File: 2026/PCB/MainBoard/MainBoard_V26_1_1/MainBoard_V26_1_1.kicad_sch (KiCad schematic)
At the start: 87 parts, among them J1 Raspberry_Pi_2_3, J13 //Drib, J15 TFT3, J16 CAN_CON, J2 fan, J4 metor, J6 Debug, J8 MOLEX MINISPOX, Q1 Q_NMOS_GSD, Q2 Q_NMOS_GSD, SW1 SW_MEC_5E, SW2 Ras_1, SW3 Ras_2, SW4 SW_Wuerth_450301014042, SW5 SW_MEC_5E, SW6 SW_MEC_5E, U1 STM32F446RETx, U10 MPU9250, U2 LMR51460FSQDRRRQ1, U3 MOUDLE-SEEEDUINO-XIAO, U5 MCP1703AT-3302E/CB, U6 BNO055, U8 MAX3051, Y1 CSTNE16M0V530000R0

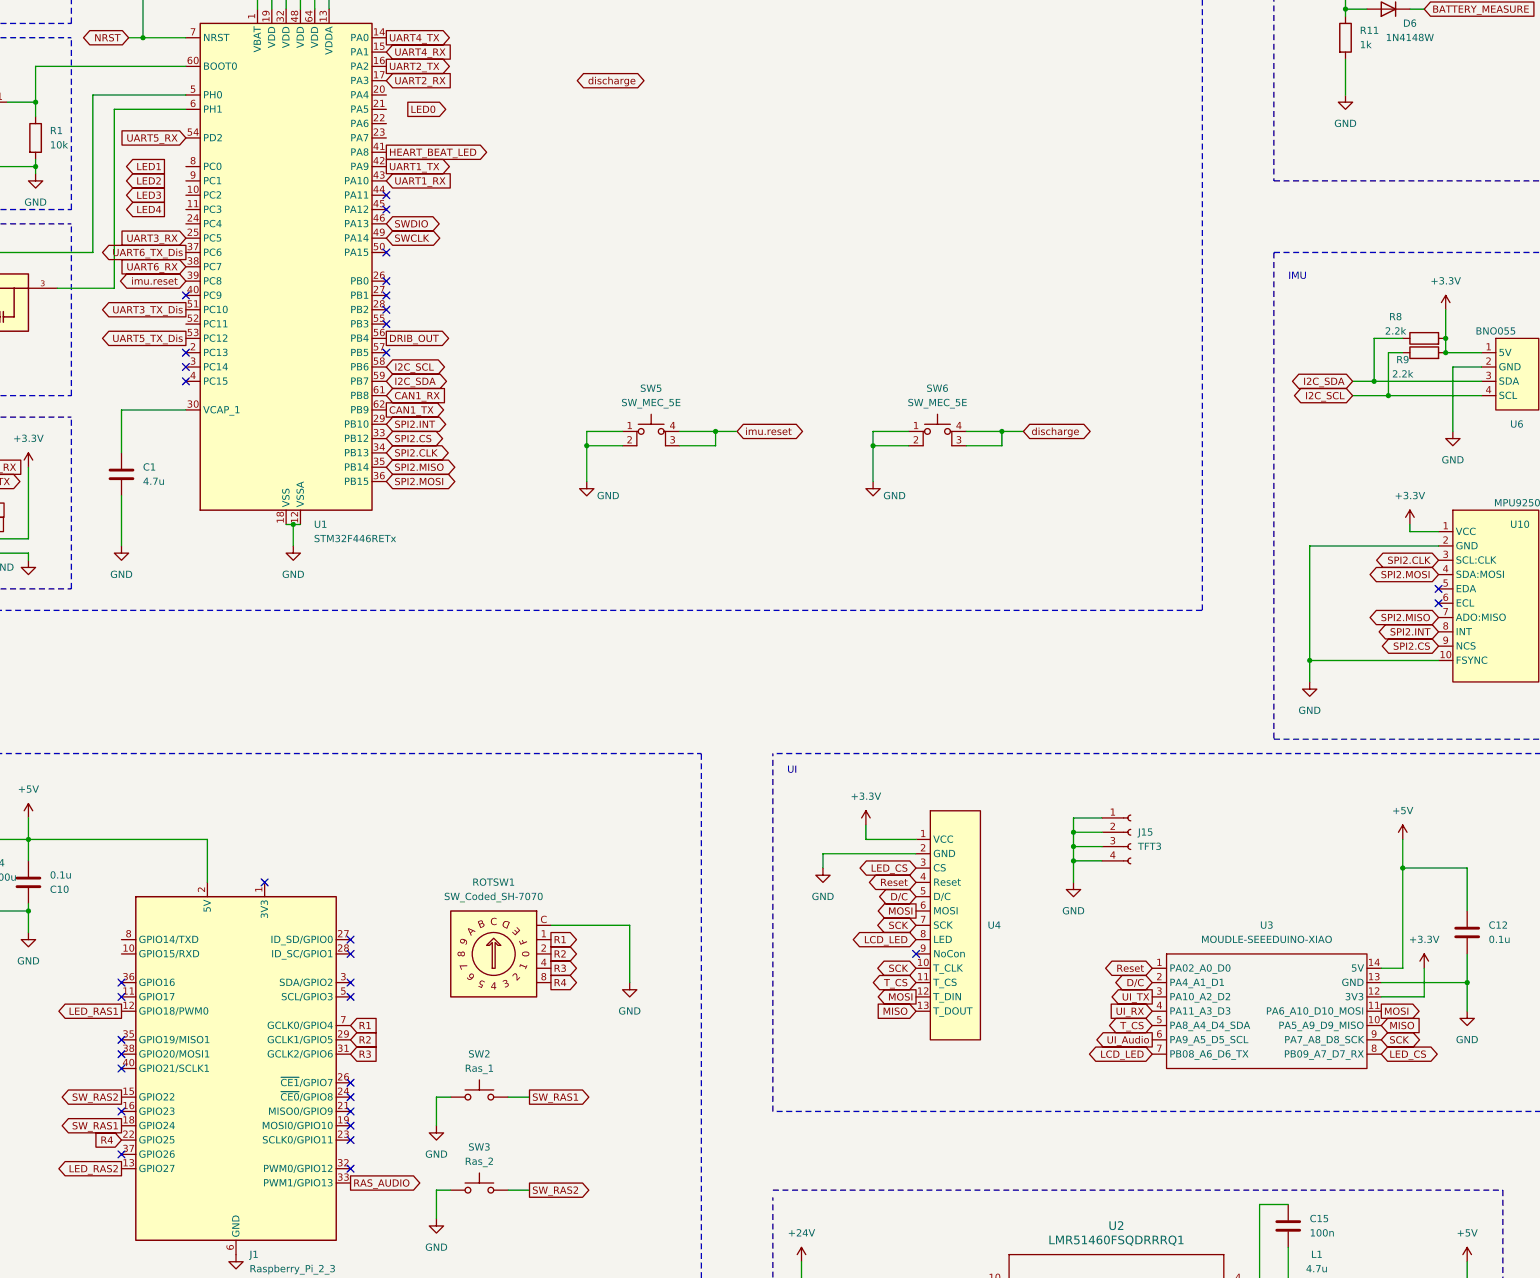
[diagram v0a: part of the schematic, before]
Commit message: 通信回りたぶん完成2
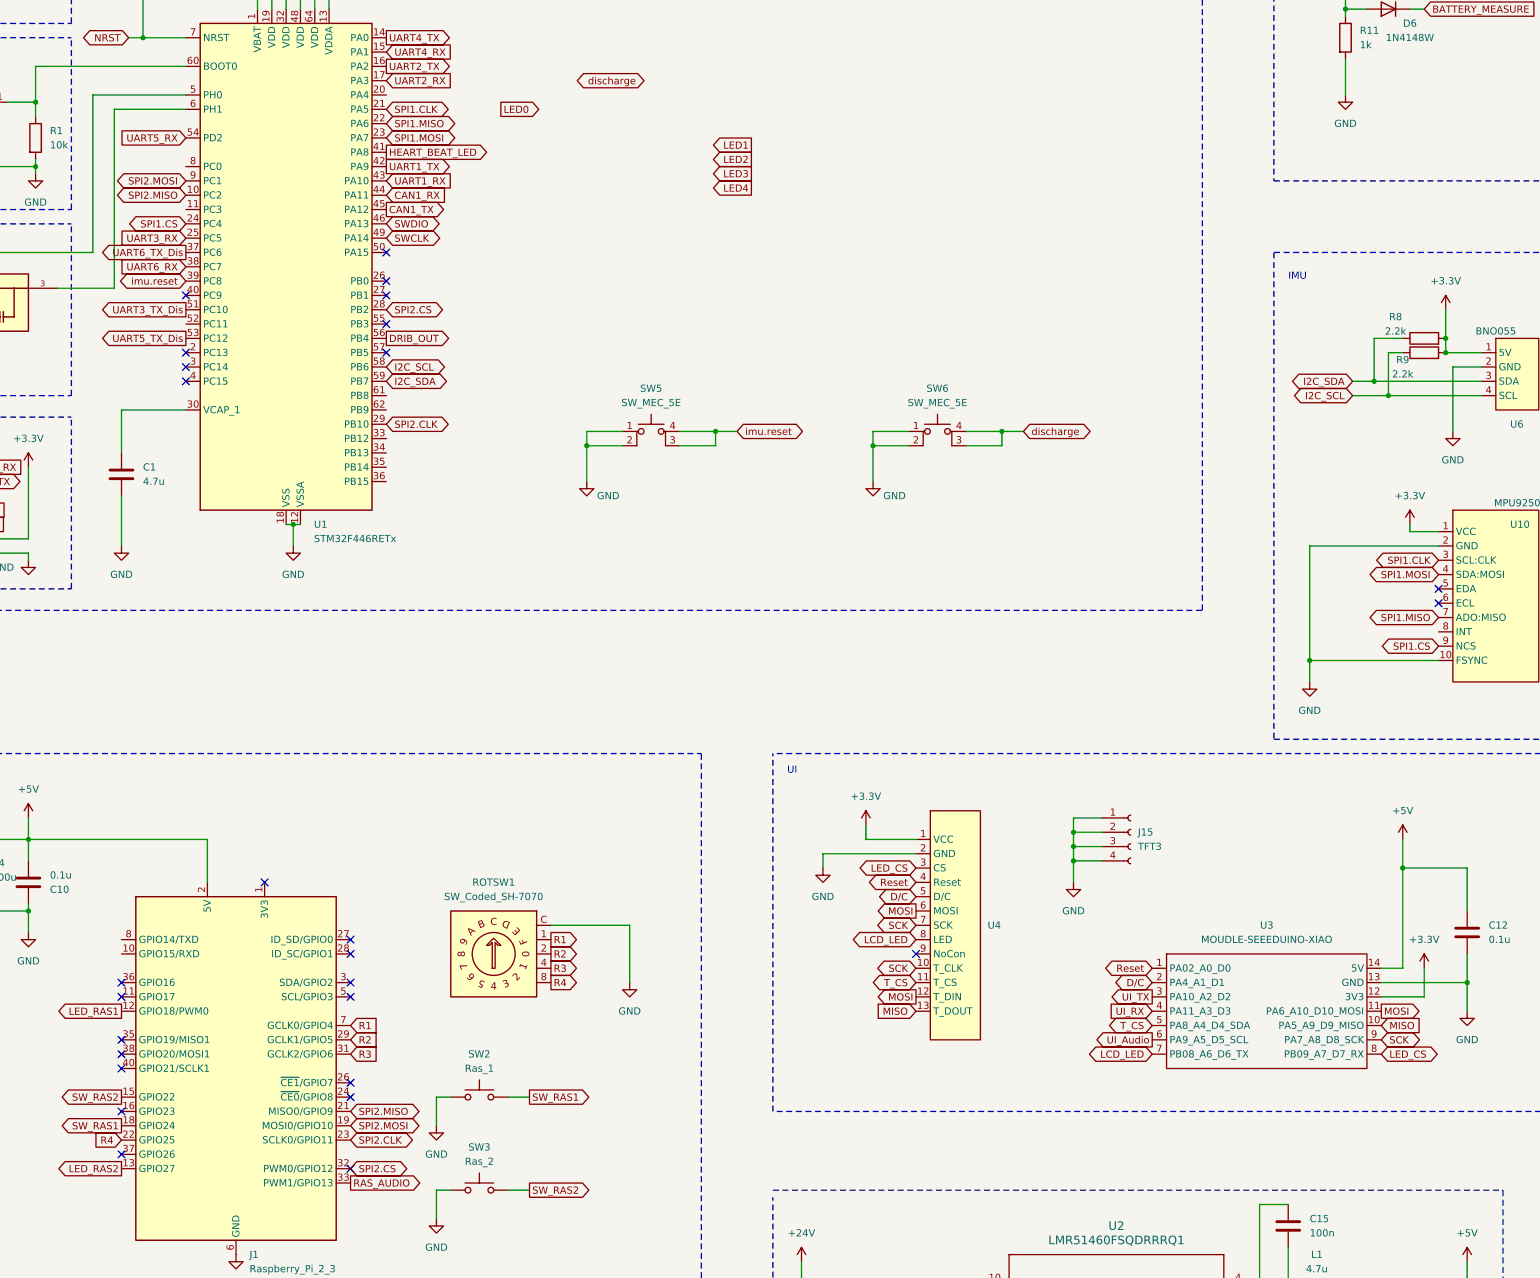
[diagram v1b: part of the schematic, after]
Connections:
- net CAN1_RX: now also U1.44 (PA11); no longer U1.61 (PB8)
- net CAN1_TX: now also U1.45 (PA12); no longer U1.62 (PB9)
- net SPI2.CLK: now also J1.23 (SCLK0/GPIO11), U1.29 (PB10); no longer U1.34 (PB13), U10.3 (SCL:CLK)
- net SPI2.CS: now also J1.32 (PWM0/GPIO12), U1.28 (PB2); no longer U1.33 (PB12), U10.9 (NCS)
- net SPI2.MISO: now also J1.21 (MISO0/GPIO9), U1.10 (PC2); no longer U1.35 (PB14), U10.7 (ADO:MISO)
- net SPI2.MOSI: now also J1.19 (MOSI0/GPIO10), U1.9 (PC1); no longer U1.36 (PB15), U10.4 (SDA:MOSI)
- net SPI1.CLK: now reaches U1.21 (PA5)
- net SPI1.CLK: now also U10.3 (SCL:CLK)
- net SPI1.MISO: now reaches U1.22 (PA6)
- net SPI1.MISO: now also U10.7 (ADO:MISO)
- net SPI1.MOSI: now reaches U1.23 (PA7)
- net SPI1.MOSI: now also U10.4 (SDA:MOSI)
- net SPI1.CS: now reaches U1.24 (PC4)
- net SPI1.CS: now also U10.9 (NCS)
- net SPI2.INT: no longer names the net of U10.8 (INT)
- net SPI2.INT: no longer U1.29 (PB10)
- no-connect marks 33 -> 27
